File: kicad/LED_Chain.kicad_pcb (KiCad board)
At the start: 2 copper layers, 63.6 x 31.5 mm, 33 parts, among them J1 Interface, J2 PWR, J3 NeoPixel R1 A, J4 NeoPixel R1 B, J5 NeoPixel R1 C, J6 NeoPixel R1 D, J7 LED, Q1 IRLML2502, Q2 IRLML2502, Q3 IRLML2502, Q4 IRLML2502, U1 HCF4027B, U2 74LS04

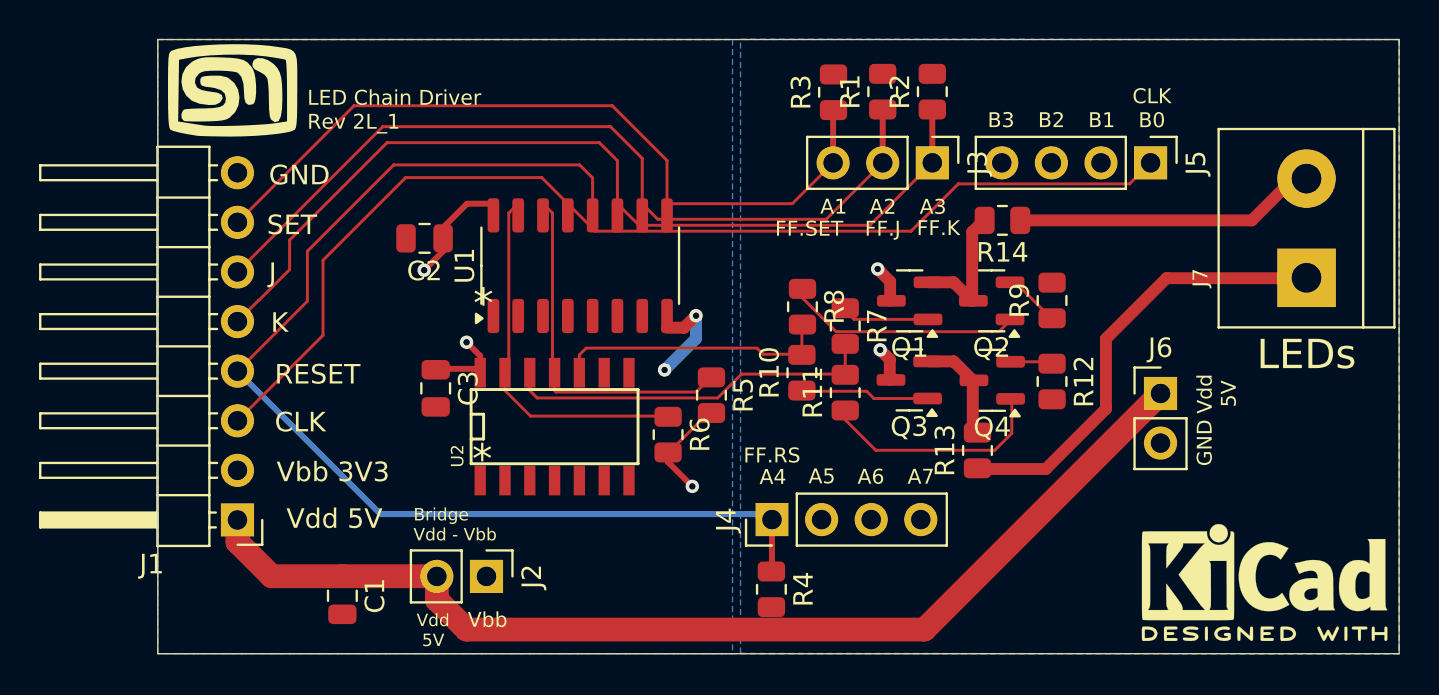
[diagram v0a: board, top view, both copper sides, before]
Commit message: Updated for V8 KiCad
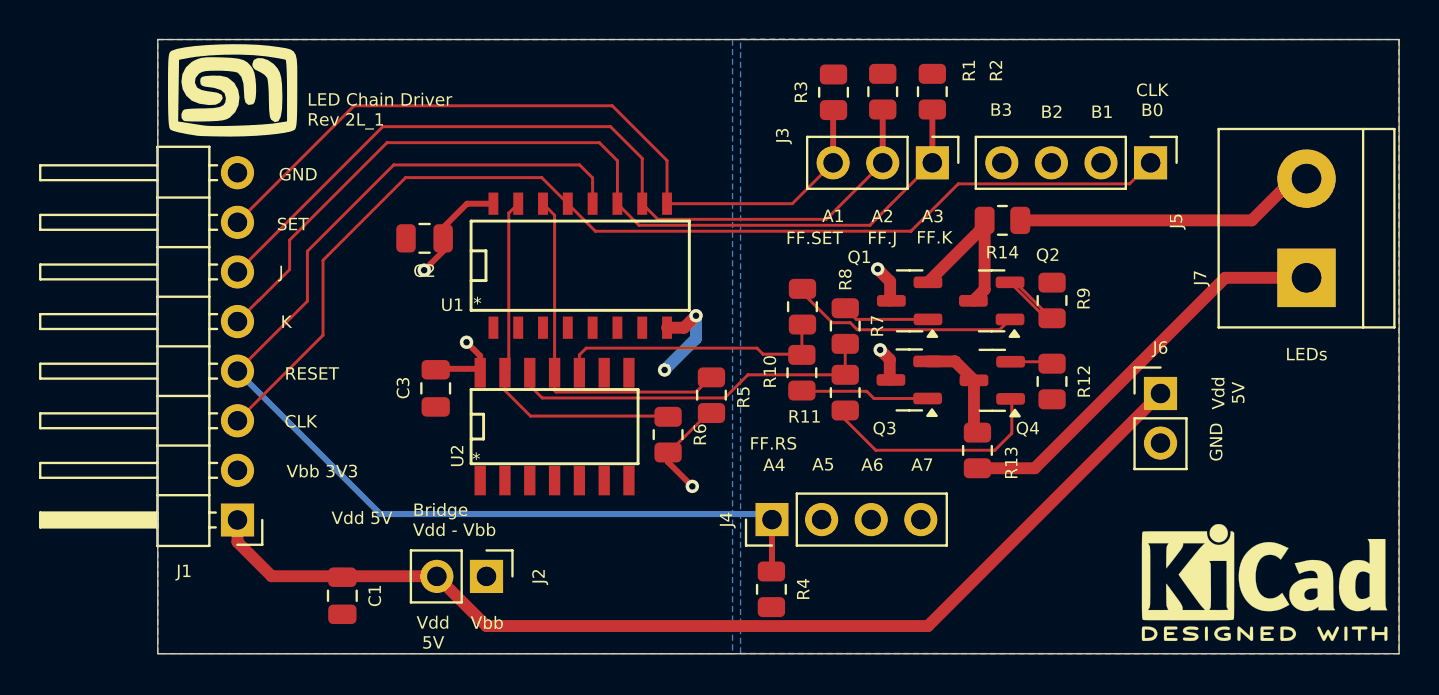
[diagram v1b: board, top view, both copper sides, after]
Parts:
- U1: footprint Package_SO:SO-16_3.9x9.9mm_P1.27mm -> LED_Chain:SO-16-N
- turned U1 to 0 degrees
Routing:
- net Net-(Q2-S): track 2.87 -> 5.78 mm
- net /LED1: track 23.5 -> 20.9 mm
- net /L2: track 6.96 -> 8.73 mm
- net /5V: track 59.6 -> 58.7 mm
